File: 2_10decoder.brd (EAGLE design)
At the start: 160 x 100 mm, 95 parts, among them T1 BC847, T10 BC847, T11 BC847, T12 BC847, T13 BC847, T14 BC847, T15 BC847, T16 BC847, T17 BC847, T18 BC847, T19 BC847, T2 BC847, T20 BC847, T21 BC847, T22 BC847, T23 BC847, T25 BC847, T3 BC847, T4 BC847, T5 BC847, T6 BC847, T7 BC847, T8 BC847, T9 BC847

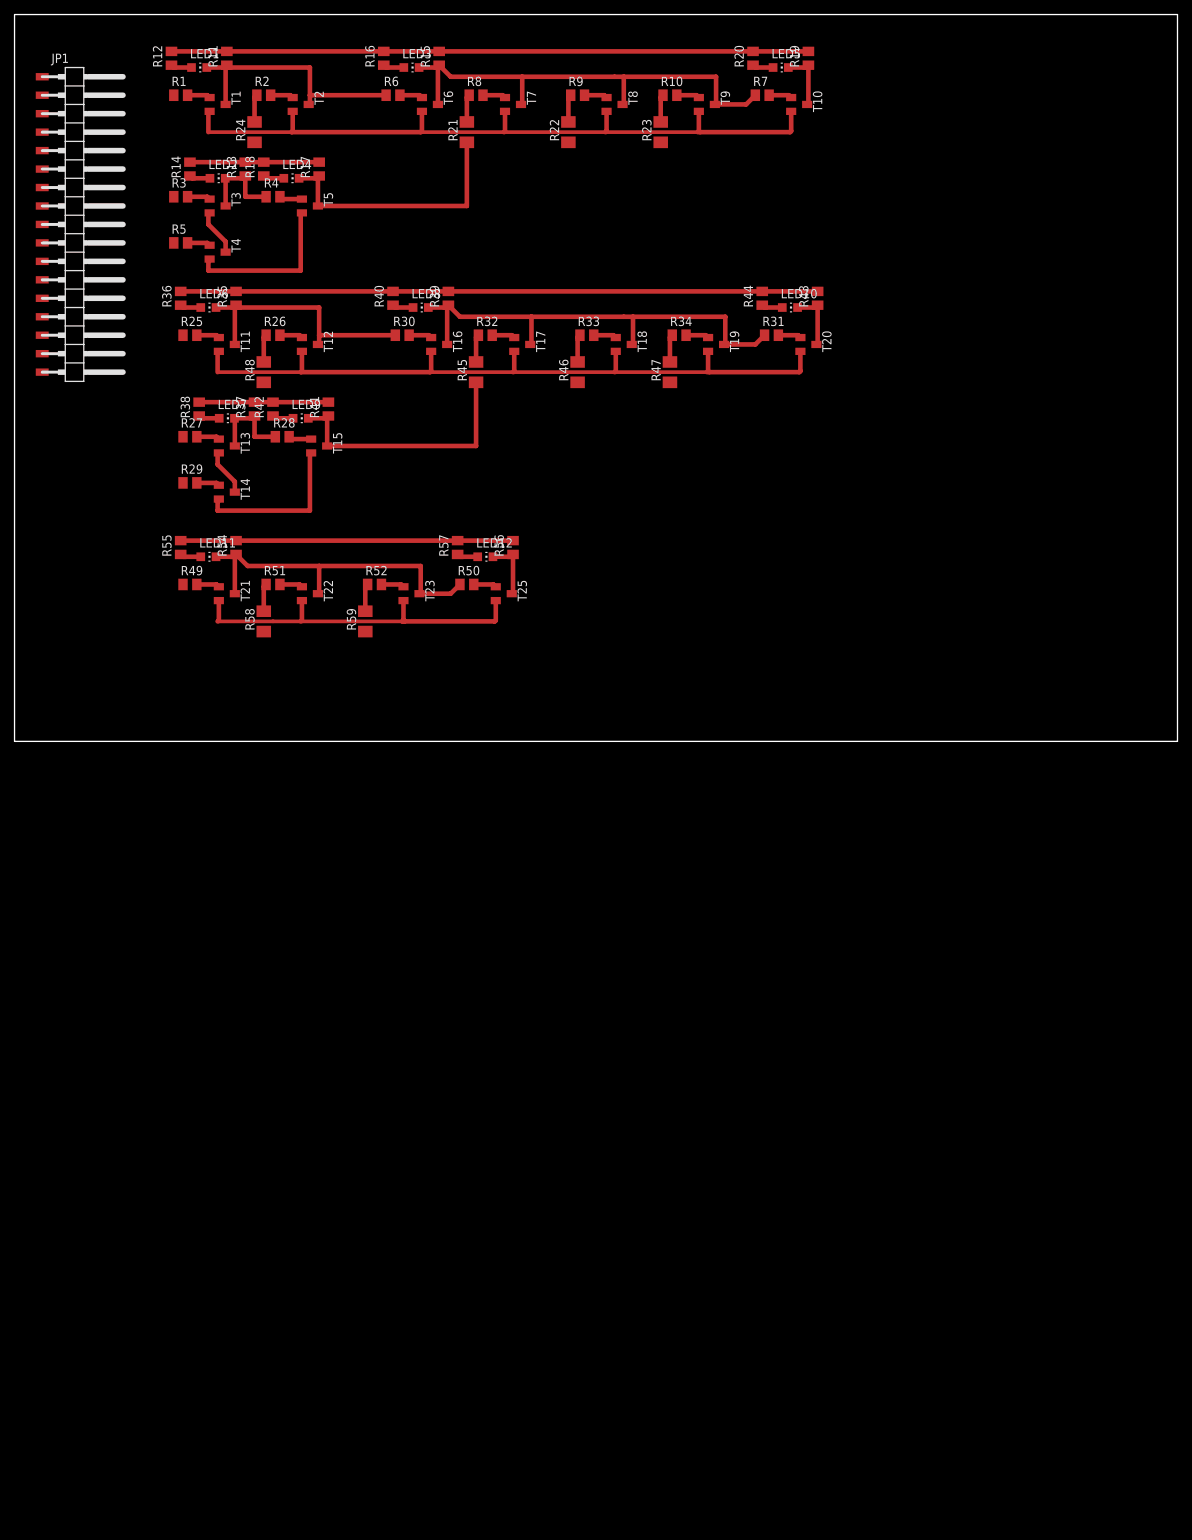
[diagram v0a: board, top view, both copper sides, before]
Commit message: final version of 2_10Decoder
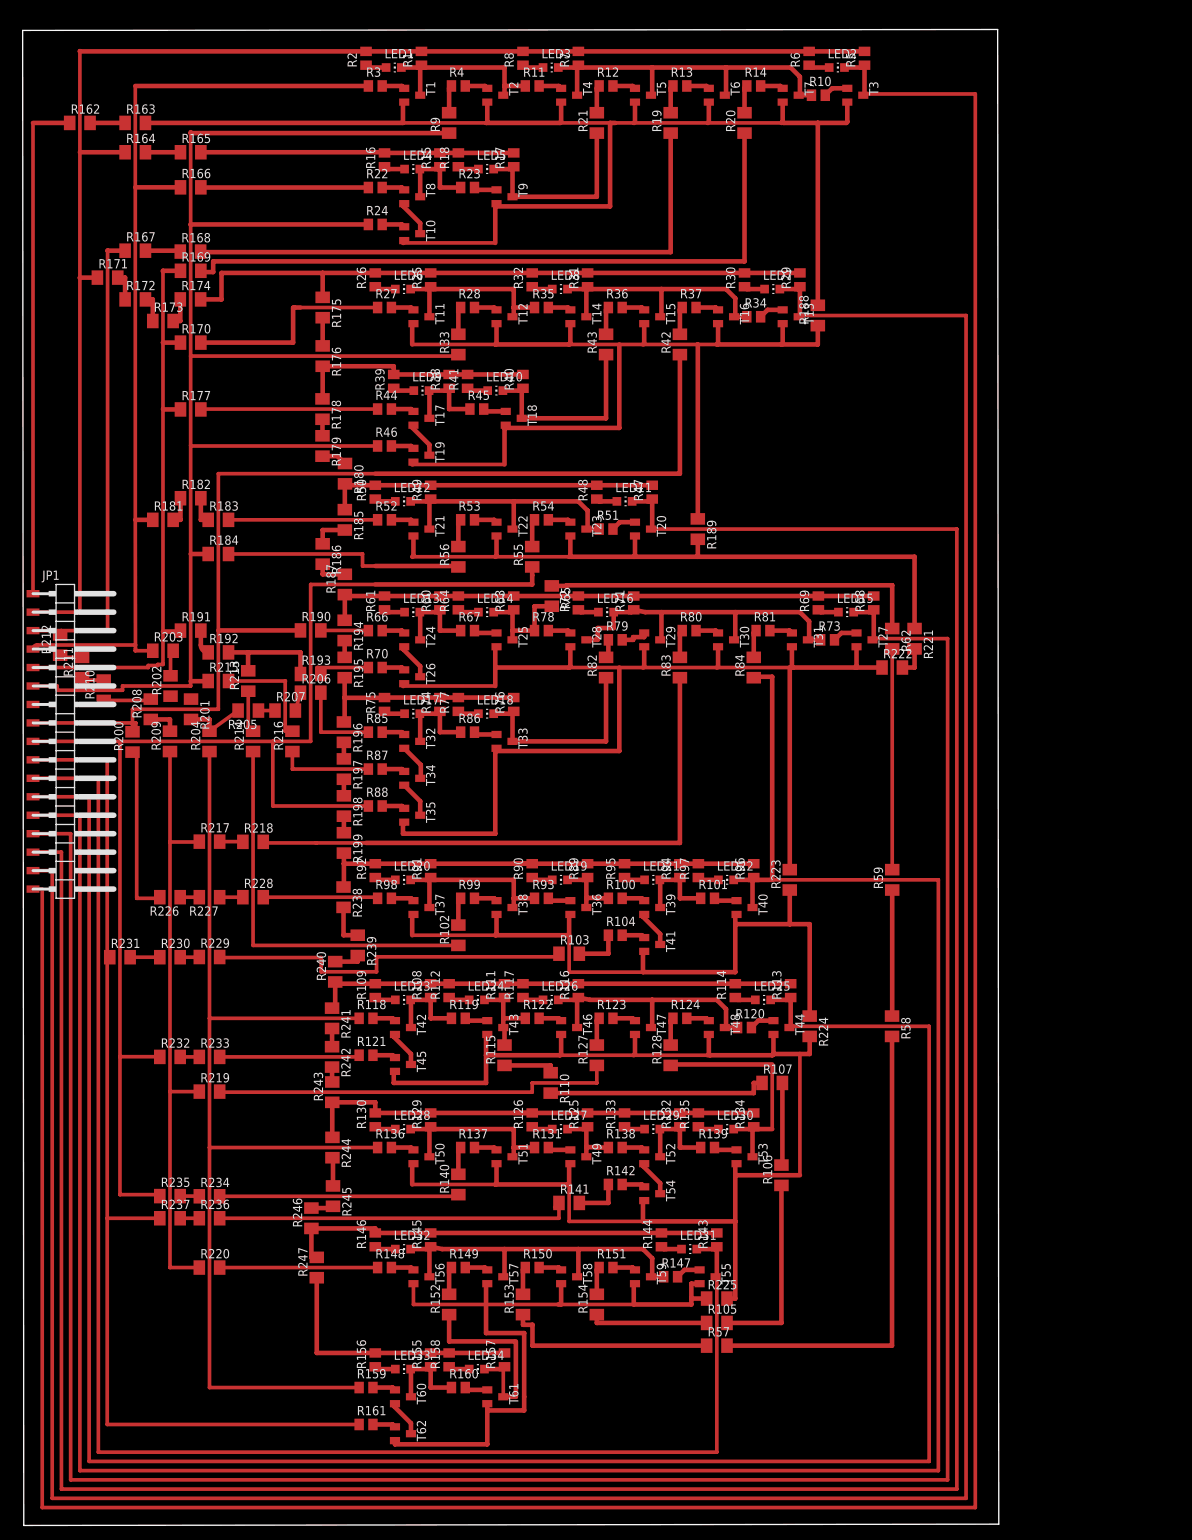
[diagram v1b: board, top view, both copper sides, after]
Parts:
- added LED13, LED14, LED15, LED16, LED17, LED18, LED19, LED20, LED21, LED22, LED23, LED24, LED25, LED26, LED27, LED28, LED29, LED30, LED31, LED32, LED33, LED34: (no value), led:CHIP-LED0805
- added R100, R101, R104, R118, R119, R120, R121, R122, R123, R124, R131, R136, R137, R138, R139, R142, R147, R148, R149, R150, R151, R159, R160, R161, R53, R66, R67, R70, R73, R78, R79, R80, R81, R85, R86, R87, R88, R93, R98, R99: 10k, resistor:M0805
- added R102, R103, R105, R106, R107, R110, R115, R127, R128, R140, R141, R152, R153, R154, R162, R163, R164, R165, R166, R167, R168, R169, R170, R171, R172, R173, R174, R175, R176, R177, R178, R179, R180, R181, R182, R183, R184, R185, R186, R187, R188, R189, R190, R191, R192, R193, R194, R195, R196, R197, R198, R199, R200, R201, R202, R203, R204, R205, R206, R207, R208, R209, R210, R211, R212, R213, R214, R215, R216, R217, R218, R219, R220, R221, R222, R223, R224, R225, R226, R227, R228, R229, R230, R231, R232, R233, R234, R235, R236, R237, R238, R239, R240, R241, R242, R243, R244, R245, R246, R247, R62, R65, R82, R83, R84: (no value), rcl:M1206
- added R108, R111, R113, R116, R125, R129, R132, R134, R143, R145, R155, R157, R60, R63, R68, R71, R74, R76, R89, R91, R94, R96: 3K9, resistor:M0805
- added R109, R112, R114, R117, R126, R130, R133, R135, R144, R146, R156, R158, R61, R64, R69, R72, R75, R77, R90, R92, R95, R97: (no value), resistor:M0805
- added T24, T26, T27, T28, T29, T30, T31, T32, T33, T34, T35, T36, T37, T38, T39, T40, T41, T42, T43, T44, T45, T46, T47, T48, T49, T50, T51, T52, T53, T54, T55, T56, T57, T58, T59, T60, T61, T62: BC847, transistor-neu-to92:SOT23
- R1, R25, R29, R31, R49, R5, R7: value 10k -> 3K9
- R11, R13, R35, R37, R54: value 3K9 -> 10k
- R12, R14, R36, R44: value (none) -> 10k
- R19, R43, R56: value 3K9 -> (none); device resistor:M0805 -> rcl:M1206
- R2, R26, R30, R32, R50, R6, R8: value 10k -> (none)
- R20, R42, R55, R57: device resistor:M0805 -> rcl:M1206
- R22, R23, R24, R45, R46: value (none) -> 10k; device rcl:M1206 -> resistor:M0805
- R33, R9: value 10k -> (none); device resistor:M0805 -> rcl:M1206
- R38, R40: value (none) -> 3K9
- R39, R41: value 3K9 -> (none)
- R47: value (none) -> 3K9; device rcl:M1206 -> resistor:M0805
- R48: device rcl:M1206 -> resistor:M0805
- moved R57 115.5 mm to (96.6, -83.1), turned to 0 degrees
- moved R58 102.8 mm to (120.7, -39.2), turned to 270 degrees
- moved R5 97.5 mm to (116.9, 94.0), turned to 90 degrees
- moved T3 89.0 mm to (115.7, 88.9)
- moved R29 88.5 mm to (108.1, 63.5), turned to 90 degrees
- moved LED2 86.5 mm to (113.1, 92.7)
- moved R59 80.7 mm to (120.8, -19.1)
- moved T13 79.6 mm to (106.8, 58.4)
- moved R14 78.4 mm to (101.7, 90.2), turned to 0 degrees
- moved LED7 77.1 mm to (104.2, 62.2)
- moved JP1 71.1 mm to (7.62, 19.1)
- moved R37 61.4 mm to (92.8, 59.7), turned to 0 degrees
- moved R13 60.9 mm to (91.5, 90.2), turned to 0 degrees
- moved R12 59.9 mm to (81.4, 90.2), turned to 0 degrees
- moved R36 59.8 mm to (82.7, 59.7), turned to 0 degrees
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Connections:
- new net G_IN1: R153.1, R57.1
- new net G_IN2: R105.1, R154.1
- new net N$100: LED26.A, R117.1
- new net N$101: R98.2, T37.1
- new net N$102: R99.2, T38.1
- new net N$103: LED20.A, R92.1
- new net N$104: LED20.C, R91.1, R93.1, T37.3, T38.3
- new net N$105: LED26.C, R116.1, R120.1, T46.3, T47.3, T48.3
- new net N$106: LED25.A, R114.1
- new net N$107: R93.2, T36.1
- new net N$108: R100.2, T39.1
- new net N$109: LED19.A, R90.1
- new net N$110: R175.2, R176.1
- new net N$111: R101.2, T40.1
- new net N$112: R178.2, R179.1
- new net N$113: R181.2, R182.1
- new net N$114: R124.1, R128.2
- new net N$115: R123.1, R127.2
- new net N$116: R185.2, R186.1
- new net N$117: R191.2, R192.1
- new net N$118: R121.2, T45.1
- new net N$119: LED17.C, R74.1, R86.1, T32.3
- new net N$120: R194.2, R195.1
- new net N$121: LED23.A, R109.1
- new net N$122: R196.2, R197.1
- new net N$123: R198.2, R199.1
- new net N$124: R238.2, R239.1
- new net N$125: T42.2, T45.3
- new net N$126: R241.2, R242.1
- new net N$127: R104.2, T41.1
- new net N$128: R244.2, R245.1
- new net N$129: LED21.C, R101.1, R94.1, T39.3
- new net N$132: R136.2, T50.1
- new net N$139: R102.2, R99.1
- new net N$141: R131.2, T49.1
- new net N$143: R138.2, T52.1
- new net N$144: LED19.C, R100.1, R89.1, T36.3
- new net N$145: T39.2, T41.3
- new net N$147: LED21.A, R95.1
- new net N$148: R139.2, T53.1
- new net N$151: LED29.C, R132.1, R139.1, T52.3
- new net N$152: T52.2, T54.3
- new net N$153: LED27.C, R125.1, R138.1, T49.3
- new net N$157: R147.2, T55.1
- new net N$158: R149.2, T57.1
- new net N$159: R150.2, T58.1
- new net N$160: R151.2, T59.1
- new net N$162: R150.1, R153.2
- new net N$164: R149.1, R152.2
- new net N$166: R151.1, R154.2
- new net N$168: R160.2, T61.1
- new net N$169: R161.2, T62.1
- new net N$173: T60.2, T62.3
- new net N$200: R66.2, T24.1
- new net N$251: LED28.A, R130.1
- new net N$252: LED28.C, R129.1, R131.1, T50.3, T51.3
- new net N$253: LED27.A, R126.1
- new net N$254: LED29.A, R133.1
- new net N$255: LED30.C, R128.1, R134.1, T53.3
- new net N$256: LED32.A, R146.1
- new net N$257: LED32.C, R145.1, R147.1, T56.3, T57.3, T58.3, T59.3
- new net N$258: LED31.A, R144.1
- new net N$260: LED33.A, R156.1
- new net N$261: LED33.C, R155.1, R160.1, T60.3
- new net N$262: LED34.C, R152.1, R157.1, T61.3
- new net N$263: R120.2, T44.1
- new net N$264: R118.2, T42.1
- new net N$265: R124.2, T48.1
- new net N$266: LED23.C, R108.1, R119.1, T42.3
- new net N$267: R119.2, T43.1
- new net N$269: R148.2, T56.1
- new net N$271: R137.1, R140.2
- new net N$272: R137.2, T51.1
- new net N$274: R142.2, T54.1
- new net N$61: R78.2, T28.1
- new net N$62: R73.2, T27.1
- new net N$65: R79.2, T29.1
- new net N$69: R80.2, T30.1
- new net N$71: R81.2, T31.1
- new net N$72: R164.2, R165.1
- new net N$73: LED16.A, R72.1
- new net N$74: LED16.C, R71.1, R73.1, T28.3, T29.3, T30.3, T31.3
- new net N$75: R85.2, T32.1
- new net N$76: LED15.A, R69.1
- new net N$77: R167.2, R168.1
- new net N$78: R80.1, R83.2
- new net N$79: R81.1, R84.2
- new net N$80: R79.1, R82.2
- new net N$81: T34.2, T35.3
- new net N$82: R67.2, T25.1
- new net N$83: R70.2, T26.1
- new net N$84: LED13.A, R61.1
- new net N$85: LED13.C, R60.1, R67.1, T24.3
- new net N$86: LED14.A, R64.1
- new net N$87: R86.2, T33.1
- new net N$88: T24.2, T26.3
- new net N$89: R122.2, T46.1
- new net N$90: R171.2, R172.1
- new net N$91: R87.2, T34.1
- new net N$92: LED17.A, R75.1
- new net N$93: R123.2, T47.1
- new net N$94: LED18.A, R77.1
- new net N$95: T32.2, T34.3
- new net N$96: R159.2, T60.1
- new net N$97: R173.2, R174.1
- new net N$98: LED18.C, R76.1, R82.1, T33.3
- new net N$99: R88.2, T35.1
- new net S$123: LED24.C, R111.1, R115.2, R122.1, T43.3
- new net S$124: LED14.C, R63.1, R65.2, R78.1, T25.3
- new net S$2: LED22.A, R97.1
- new net S$4: LED24.A, R112.1
- new net S$40: LED30.A, R135.1
- new net S$5: LED34.A, R158.1
- net !T: now also R103.1, R141.1, R161.1, R229.1, R229.2, R230.1, R230.2, R231.1, R231.2, R236.1, R236.2, R237.1, R237.2
- net !Y: now also R190.1, R190.2, R200.1, R200.2, R226.1, R226.2, R227.1, R227.2, R228.1, R228.2, R42.1, R66.1, R98.1
- net !Z: now also R121.1, R140.1, R232.1, R232.2, R233.1, R233.2, R234.1, R234.2, R235.1, R235.2, R55.1, R88.1
- net A: now also JP1.17, LED2.C, R5.1, T3.3; no longer JP1.11
- net B: now also JP1.16, LED7.C, R29.1, T13.3; no longer JP1.12
- net C: now also JP1.15, LED11.C, R47.1, T20.3; no longer JP1.13
- net D: now also LED15.C, R68.1, T27.3
- net E: now also JP1.13, LED22.C, R84.1, R96.1, T40.3; no longer JP1.15
- net F: now also JP1.12, LED25.C, R113.1, T44.3; no longer JP1.16
- net G: now also JP1.11, LED31.C, R143.1, T55.3; no longer JP1.17
- net GND: now also R162.1, R163.2, R188.1, R188.2, R189.1, R189.2, R221.1, R221.2, R222.1, R222.2, R223.1, R223.2, R224.1, R224.2, R225.1, R225.2, T13.2, T26.2, T27.2, T28.2, T29.2, T3.2, T30.2, T31.2, T33.2, T35.2, T36.2, T37.2, T38.2, T40.2, T41.2, T43.2, T44.2, T45.2, T46.2, T47.2, T48.2, T49.2, T50.2, T51.2, T53.2, T54.2, T55.2, T56.2, T57.2, T58.2, T59.2, T61.2, T62.2; no longer T17.2, T8.2
- net N$1: now also LED4.A, R16.1; no longer LED2.A, R14.1
- net N$10: now also R12.2, T5.1; no longer R8.2, T7.1
- net N$11: now also R13.2, T6.1; no longer R9.2, T8.1
- net N$12: now also R14.2, T7.1; no longer R10.2, T9.1
- net N$13: now also R2.1; no longer R12.1
- net N$14: now also R1.1; no longer R6.1
- net N$15: now also R4.1, R9.2; no longer R2.1, R24.2
- net N$16: now also R103.2, R104.1; no longer R1.1
- net N$17: now also R8.1; no longer R16.1
- net N$18: now also R10.1, T4.3, T5.3; no longer R15.1, T8.3, T9.3
- net N$19: now also LED5.A; no longer LED4.A
- net N$2: now also LED4.C, R15.1, R23.1, T8.3; no longer LED2.C, R13.1, R4.1, T3.3
- net N$20: now also LED5.C, T9.3; no longer LED4.C, T5.3
- net N$21: now also LED2.A, R6.1; no longer LED5.A, R20.1
- net N$22: now also R141.2, R142.1; no longer LED5.C, R19.1, T10.3
- net N$23: now also T10.3, T8.2; no longer T3.2, T4.3
- net N$24: now also R12.1; no longer R8.1
- net N$25: now also R106.2, R107.2; no longer R3.1
- net N$26: now also R110.1, R115.1; no longer R5.1
- net N$27: now also R27.2; no longer R25.2
- net N$28: now also R28.2; no longer R26.2
- net N$29: now also R13.1, R19.2; no longer R22.2, R9.1
- net N$3: now also R3.2; no longer R1.2
- net N$30: now also R14.1, R20.2; no longer R10.1, R23.2
- net N$31: now also R44.2, T17.1; no longer R27.2, T13.1
- net N$32: now also R45.2, T18.1; no longer R28.2, T15.1
- net N$33: now also R46.2, T19.1; no longer R29.2, T14.1
- net N$34: now also R35.2, T14.1; no longer R30.2, T16.1
- net N$35: now also R34.2, T13.1; no longer R31.2, T20.1
- net N$36: now also R36.2, T15.1; no longer R32.2, T17.1
- net N$37: now also R37.2, T16.1; no longer R33.2, T18.1
- net N$38: now also R105.2, R106.1; no longer R34.2, T19.1
- net N$39: now also R26.1; no longer R36.1
- net N$4: now also R4.2; no longer R2.2
- net N$40: now also R25.1; no longer R30.1
- net N$41: now also R28.1, R33.2; no longer R26.1, R48.2
- net N$42: now also R107.1, R110.2; no longer R25.1
- net N$43: now also LED9.A, R39.1; no longer LED7.A, R38.1
- net N$44: now also LED9.C, R38.1, R45.1, T17.3; no longer LED7.C, R28.1, R37.1, T13.3
- net N$45: now also R32.1; no longer R40.1
- net N$46: now also R34.1, T14.3, T15.3; no longer R39.1, T17.3, T18.3, T19.3
- net N$47: now also LED10.A, R41.1; no longer LED9.A, R42.1
- net N$48: now also LED10.C, R40.1, R43.1, T18.3; no longer LED9.C, R41.1, R45.1, T15.3
- net N$49: now also LED7.A, R30.1; no longer LED10.A, R44.1
- net N$5: now also R22.2, T8.1; no longer R3.2, T3.1
- net N$50: now also R62.1, R65.1; no longer LED10.C, R43.1, T20.3
- net N$51: now also T17.2, T19.3; no longer T13.2, T14.3
- net N$52: now also R59.2, R62.2; no longer R27.1
- net N$53: now also R58.1, R59.1; no longer R29.1
- net N$54: now also R37.1, R42.2; no longer R33.1, R46.2
- net N$55: now also R57.2, R58.2; no longer R34.1, R47.2
- net N$56: now also R36.1, R43.2; no longer R32.1, R45.2
- net N$57: now also R52.2; no longer R49.2
- net N$58: now also R51.2, T20.1; no longer R50.2, T25.1
- net N$59: now also R53.2; no longer R51.2
- net N$6: now also R23.2, T9.1; no longer R4.2, T5.1
- net N$60: now also R54.2; no longer R52.2
- net N$63: now also LED12.A, R50.1; no longer LED11.A, R55.1
- net N$64: now also LED12.C, R49.1, R51.1; no longer LED11.C, R50.1, R54.1
- net N$66: now also LED11.A, R48.1; no longer LED12.A, R57.1
- net N$67: now also R162.2, R163.1; no longer LED12.C, R56.1, T25.3
- net N$68: now also R54.1, R55.2; no longer R52.1, R59.2
- net N$7: now also R24.2, T10.1; no longer R5.2, T4.1
- net N$70: now also R53.1, R56.2; no longer R51.1, R58.2
- net N$8: now also R11.2, T4.1; no longer R6.2, T6.1
- net N$9: now also R10.2, T3.1; no longer R7.2, T10.1
- net T: now also R184.1, R184.2, R215.1, R215.2, R216.1, R216.2, R24.1, R33.1, R46.1, R56.1, R87.1, R9.1
- net VCC: now also R1.2, R108.2, R109.2, R111.2, R112.2, R113.2, R114.2, R116.2, R117.2, R125.2, R126.2, R129.2, R130.2, R132.2, R133.2, R134.2, R135.2, R143.2, R144.2, R145.2, R146.2, R155.2, R156.2, R157.2, R158.2, R164.1, R165.2, R171.1, R172.2, R173.1, R174.2, R175.1, R176.2, R178.1, R179.2, R180.1, R180.2, R182.2, R183.1, R185.1, R186.2, R187.1, R187.2, R194.1, R195.2, R196.1, R197.2, R198.1, R199.2, R2.2, R238.1, R239.2, R240.1, R240.2, R241.1, R242.2, R243.1, R243.2, R244.1, R245.2, R246.1, R246.2, R247.1, R247.2, R25.2, R26.2, R29.2, R30.2, R31.2, R32.2, R47.2, R48.2, R49.2, R5.2, R50.2, R6.2, R60.2, R61.2, R63.2, R64.2, R68.2, R69.2, R7.2, R71.2, R72.2, R74.2, R75.2, R76.2, R77.2, R8.2, R89.2, R90.2, R91.2, R92.2, R94.2, R95.2, R96.2, R97.2; no longer R11.2, R12.2, R13.2, R14.2, R19.2, R20.2, R35.2, R36.2, R37.2, R42.2, R43.2, R44.2, R54.2, R55.2, R56.2, R57.2
- net X: now also R127.1, R148.1, R167.1, R168.2, R19.1, R208.1, R208.2, R209.1, R209.2, R210.1, R210.2, R211.1, R211.2, R212.1, R212.2, R217.1, R217.2, R218.1, R218.2, R219.1, R219.2, R220.1, R220.2, R83.1
- net Y: now also R118.1, R136.1, R159.1, R166.1, R166.2, R181.1, R183.2, R201.1, R201.2, R202.1, R202.2, R203.1, R203.2, R204.1, R204.2, R205.1, R205.2, R206.1, R206.2, R207.1, R207.2, R22.1, R3.1, R52.1, R85.1
- net Z: now also R102.1, R169.1, R169.2, R170.1, R170.2, R177.1, R177.2, R191.1, R192.2, R193.1, R193.2, R20.1, R213.1, R213.2, R214.1, R214.2, R27.1, R44.1, R70.1
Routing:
- net GND: track 295.6 -> 1054.6 mm
- net VCC: track 256.5 -> 840.8 mm
- net A: track 0.00 -> 431.6 mm
- net X: track 0.00 -> 408.4 mm
- net B: track 0.00 -> 407.4 mm
- net C: track 0.00 -> 396.0 mm
- net Y: track 0.00 -> 360.2 mm
- net E: track 0.00 -> 359.4 mm
- net D: track 0.00 -> 347.7 mm
- net Z: track 0.00 -> 314.2 mm
- net F: track 0.00 -> 300.7 mm
- net T: track 0.00 -> 288.8 mm
- net !T: track 0.00 -> 253.9 mm
- net !Z: track 0.00 -> 246.6 mm
- net G: track 0.00 -> 218.2 mm
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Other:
- board size 160 x 100 mm -> 134.3 x 205.8 mm
